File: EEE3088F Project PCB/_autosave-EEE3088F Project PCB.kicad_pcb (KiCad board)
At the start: 2 copper layers, 76 x 53 mm, 52 parts, among them IC1 74LVC1G04SE-7, J1 JST PH 2.00mm connector, J2 TYPE-C-31-M-12, SW1 SS12D07VG5 087, U1 DRV8833PWR, U10 LM7805_TO220, U11 TC4056A., U2 DRV8833PWPR, U3 INA219AxD, U4 CH224K, U5 TPS22918, U6 MIC5504-1.2YM5, U7 SX1308, U8 TPS22965DSGR, U9 TPS22965DSGR

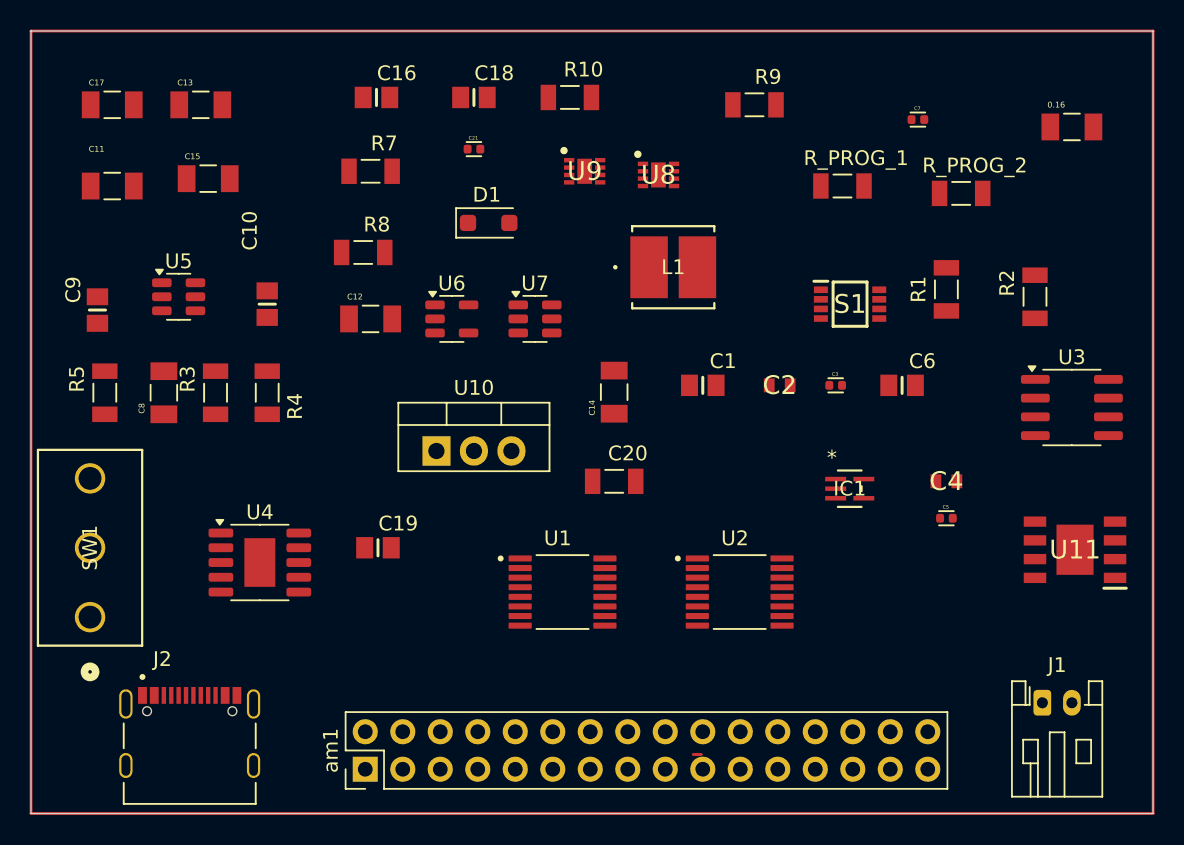
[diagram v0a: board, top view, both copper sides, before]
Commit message: finished circuit
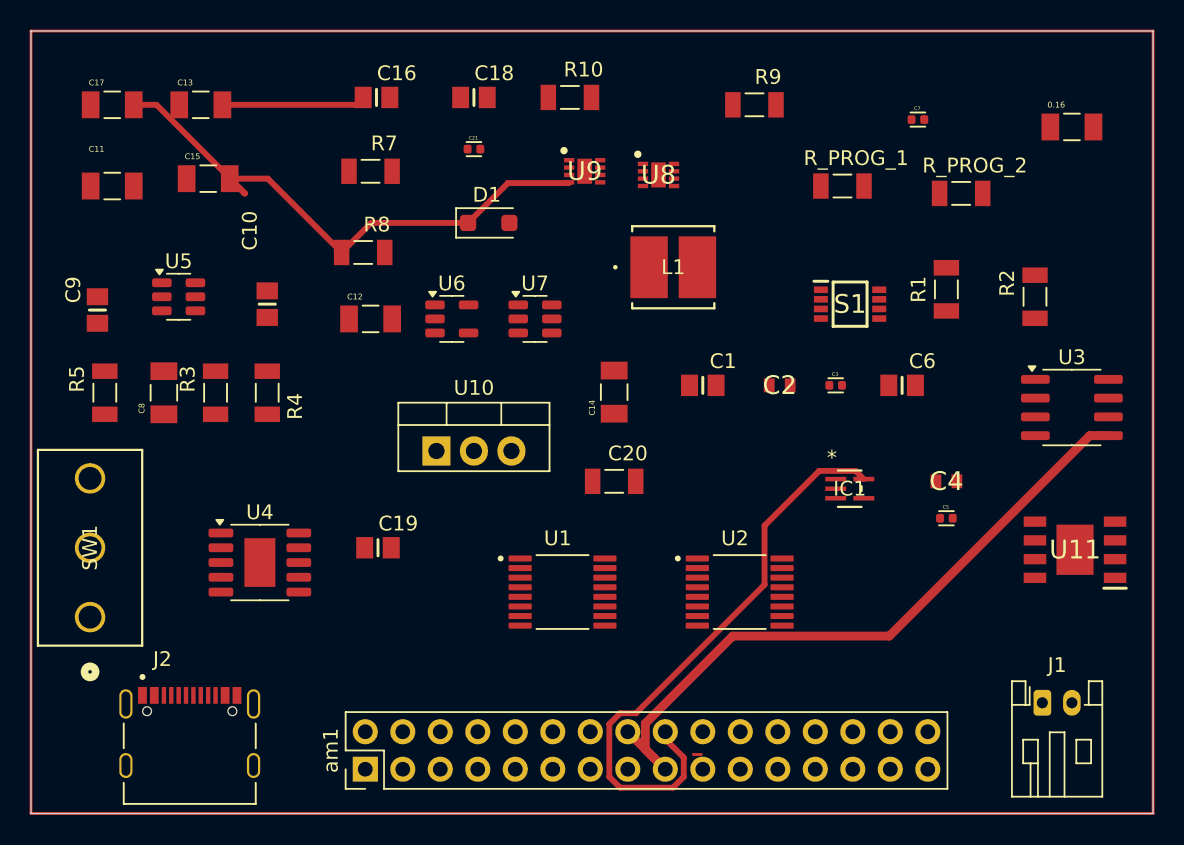
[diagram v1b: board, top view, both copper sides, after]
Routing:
- net /I2C1_SCL: track 0.00 -> 46.7 mm
- net /3V3 Out: track 0.00 -> 40.3 mm
- net /5V Out: track 0.00 -> 38.5 mm
- net GND: track 0.00 -> 9.75 mm
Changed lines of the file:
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@@
 		(layer "Edge.Cuts")
+	)
+	(segment
+		(start 170.851613 106.796614)
+		(end 171.405 107.350001)
+		(width 0.4)
+		(layer "F.Cu")
+		(net 5)
+	)
+	(segment
+		(start 159.211 127.518182)
+		(end 158.478182 128.251)
+		(width 0.4)
+		(layer "F.Cu")
+		(net 5)
+	)
+	(segment
+		(start 155.975 123.209)
+		(end 164.684 114.5)
+		(width 0.4)
+		(layer "F.Cu")
+		(net 5)
+	)
+	(segment
+		(start 157.5 124.5)
+		(end 159.211 126.211)
+		(width 0.4)
+		(layer "F.Cu")
+		(net 5)
+	)
+	(segment
+		(start 157.96 124.46)
+		(end 157.92 124.5)
+		(width 0.4)
+		(layer "F.Cu")
+		(net 5)
+	)
+	(segment
+		(start 159.211 126.211)
+		(end 159.211 127.518182)
+		(width 0.4)
+		(layer "F.Cu")
+		(net 5)
+	)
+	(segment
+		(start 158.478182 128.251)
+		(end 154.901818 128.251)
+		(width 0.4)
+		(layer "F.Cu")
+		(net 5)
+	)
+	(segment
+		(start 168.3878 106.796614)
+		(end 170.851613 106.796614)
+		(width 0.4)
+		(layer "F.Cu")
+		(net 5)
+	)
+	(segment
+		(start 164.684 114.5)
+		(end 164.684 110.500414)
+		(width 0.4)
+		(layer "F.Cu")
+		(net 5)
+	)
+	(segment
+		(start 154.901818 123.209)
+		(end 155.975 123.209)
+		(width 0.4)
+		(layer "F.Cu")
+		(net 5)
+	)
+	(segment
+		(start 154.169 123.941818)
+		(end 154.901818 123.209)
+		(width 0.4)
+		(layer "F.Cu")
+		(net 5)
+	)
+	(segment
+		(start 154.169 127.518182)
+		(end 154.169 123.941818)
+		(width 0.4)
+		(layer "F.Cu")
+		(net 5)
+	)
+	(segment
+		(start 164.684 110.500414)
+		(end 168.3878 106.796614)
+		(width 0.4)
+		(layer "F.Cu")
+		(net 5)
+	)
+	(segment
+		(start 157.92 124.5)
+		(end 157.5 124.5)
+		(width 0.4)
+		(layer "F.Cu")
+		(net 5)
+	)
+	(segment
+		(start 154.901818 128.251)
+		(end 154.169 127.518182)
+		(width 0.4)
+		(layer "F.Cu")
+		(net 5)
+	)
+	(segment
+		(start 127.96 82)
+		(end 137 82)
+		(width 0.4)
+		(layer "F.Cu")
+		(net 18)
+	)
+	(segment
+		(start 137 82)
+		(end 137.5 81.5)
+		(width 0.4)
+		(layer "F.Cu")
+		(net 18)
+	)
+	(segment
+		(start 156.609 123.900397)
+		(end 162.528397 117.981)
+		(width 0.6)
+		(layer "F.Cu")
+		(net 22)
+	)
+	(segment
+		(start 157.96 127)
+		(end 155.42 124.46)
+		(width 0.6)
+		(layer "F.Cu")
+		(net 22)
+	)
+	(segment
+		(start 173.1345 117.981)
+		(end 186.7105 104.405)
+		(width 0.6)
+		(layer "F.Cu")
+		(net 22)
+	)
+	(segment
+		(start 157.96 127)
+		(end 156.609 125.649)
+		(width 0.6)
+		(layer "F.Cu")
+		(net 22)
+	)
+	(segment
+		(start 186.7105 104.405)
+		(end 187.975 104.405)
+		(width 0.6)
+		(layer "F.Cu")
+		(net 22)
+	)
+	(segment
+		(start 162.528397 117.981)
+		(end 173.1345 117.981)
+		(width 0.6)
+		(layer "F.Cu")
+		(net 22)
+	)
+	(segment
+		(start 156.609 125.649)
+		(end 156.609 123.900397)
+		(width 0.6)
+		(layer "F.Cu")
+		(net 22)
+	)
+	(segment
+		(start 136.04 92)
+		(end 138.04 90)
+		(width 0.4)
+		(layer "F.Cu")
+		(net 27)
+	)
+	(segment
+		(start 144.6 90)
+		(end 147.299 87.301)
+		(width 0.4)
+		(layer "F.Cu")
+		(net 27)
+	)
+	(segment
+		(start 129.46 88)
+		(end 129.5 88)
+		(width 0.4)
+		(layer "F.Cu")
+		(net 27)
+	)
+	(segment
+		(start 128.46 87)
+		(end 129.46 88)
+		(width 0.4)
+		(layer "F.Cu")
+		(net 27)
+	)
+	(segment
+		(start 147.299 87.301)
+		(end 151.45 87.301)
+		(width 0.4)
+		(layer "F.Cu")
+		(net 27)
+	)
+	(segment
+		(start 129.5 88)
+		(end 123.5 82)
+		(width 0.4)
+		(layer "F.Cu")
+		(net 27)
+	)
+	(segment
+		(start 131.04 87)
+		(end 136.04 92)
+		(width 0.4)
+		(layer "F.Cu")
+		(net 27)
+	)
+	(segment
+		(start 128.46 87)
+		(end 131.04 87)
+		(width 0.4)
+		(layer "F.Cu")
+		(net 27)
+	)
+	(segment
+		(start 138.04 90)
+		(end 144.6 90)
+		(width 0.4)
+		(layer "F.Cu")
+		(net 27)
+	)
+	(segment
+		(start 123.5 82)
+		(end 121.96 82)
+		(width 0.4)
+		(layer "F.Cu")
+		(net 27)
 	)
 	(embedded_fonts no)
